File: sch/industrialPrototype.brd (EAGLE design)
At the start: 160 x 100 mm, 13 parts, among them IC1 LD1117V33C, U1 PIC16F1825-I/SL

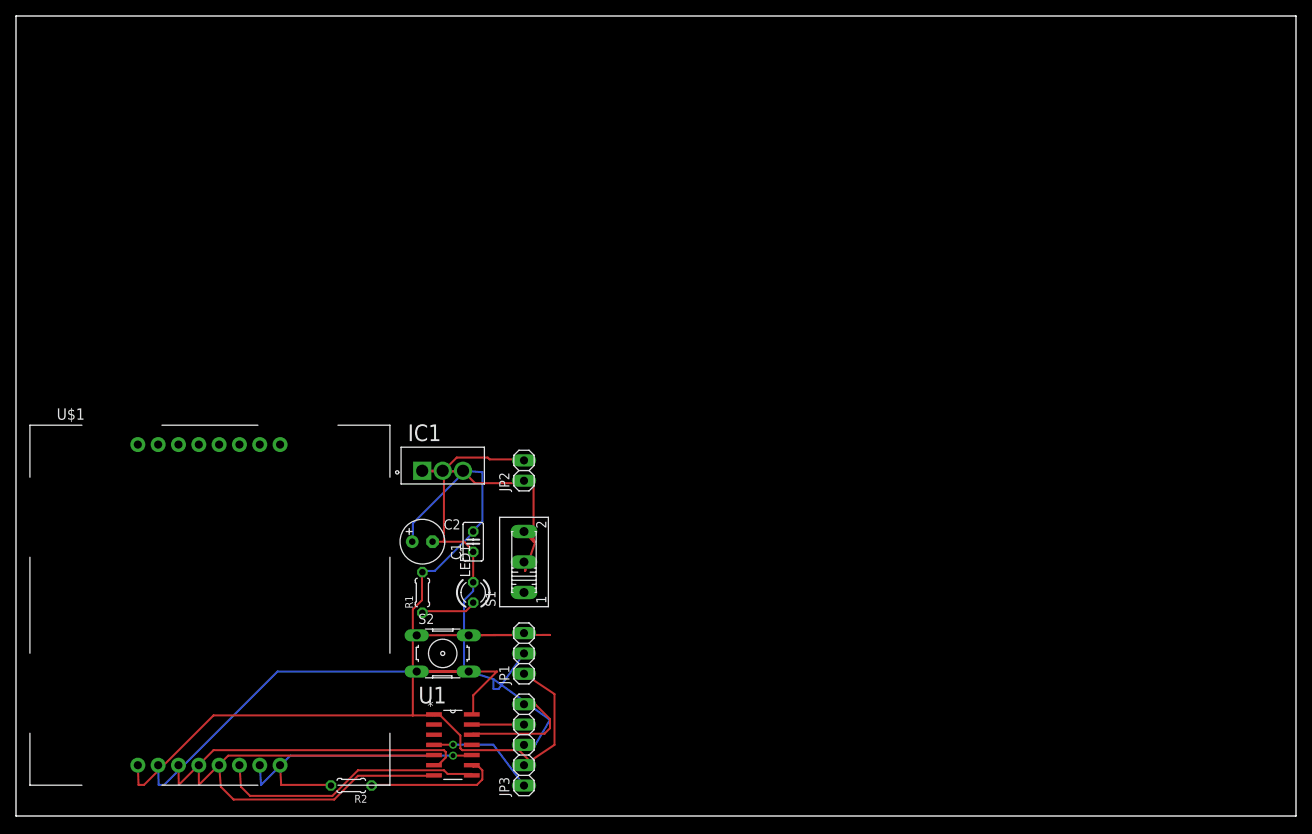
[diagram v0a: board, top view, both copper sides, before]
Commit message: Final Version of the Schematic and Board
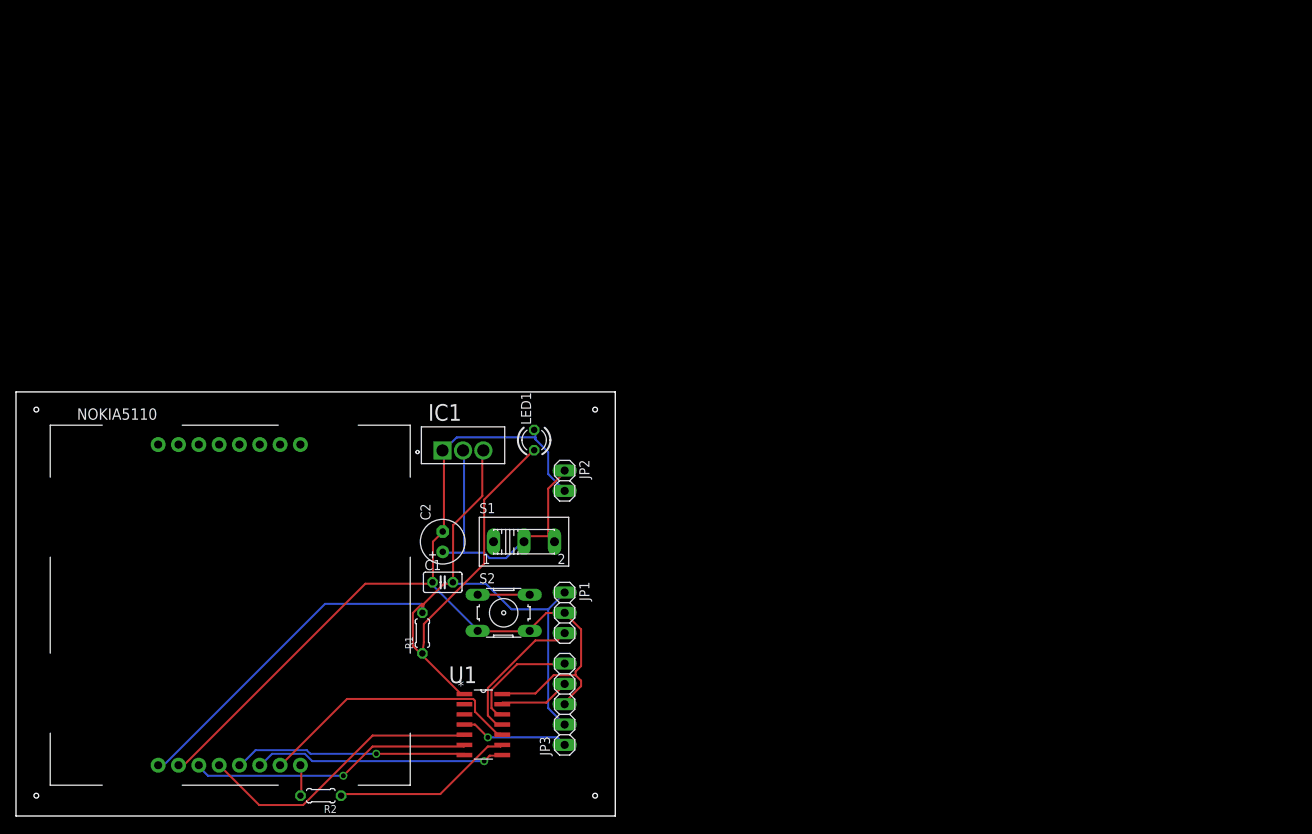
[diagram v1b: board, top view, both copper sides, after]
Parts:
- removed U$1: NOKIA5110, CustomLib:NOKIA5110
- added NOKIA5110: NOKIA5110, CustomLib:NOKIA5110
- moved LED1 20.5 mm to (64.8, 47.0)
- moved S2 9.16 mm to (61.0, 25.4)
- moved JP3 7.18 mm to (68.6, 14.0)
- moved JP1 7.18 mm to (68.6, 25.4), turned to 270 degrees
- moved C1 6.35 mm to (53.3, 29.2), turned to 0 degrees
- moved JP2 5.24 mm to (68.6, 41.9), turned to 270 degrees
- moved R1 5.08 mm to (50.8, 22.9)
- moved U1 4.58 mm to (58.4, 11.4)
- moved R2 4.02 mm to (38.1, 2.54)
- moved IC1 3.59 mm to (58.4, 47.0)
- moved C2 2.54 mm to (53.3, 34.3), turned to 90 degrees
- moved S1 2.54 mm to (63.5, 34.3), turned to 0 degrees
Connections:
- net !RST!: now also NOKIA5110.B4; no longer U$1.B4
- net !SCE!: now also NOKIA5110.B3; no longer U$1.B3
- net 3V3: now also NOKIA5110.B1; no longer U$1.B1
- net D/C: now also NOKIA5110.B5; no longer U$1.B5
- net DN(MOSI): now also NOKIA5110.B6; no longer U$1.B6
- net GND: now also NOKIA5110.B2; no longer U$1.B2
- net LED: now also NOKIA5110.B8; no longer U$1.B8
- net SCLK: now also NOKIA5110.B7; no longer U$1.B7
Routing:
- net N$1: track 6.97 -> 31.2 mm
- net !MCLK!: track 26.8 -> 6.50 mm
- net GND: track 142.4 -> 124.2 mm
- net 1WIRE_DS18B20: track 0.00 -> 18.1 mm
- net VBAT: track 44.6 -> 38.6 mm
- net N$3: track 16.9 -> 22.8 mm
- net LED: track 8.73 -> 3.87 mm
- net !SCE!: track 40.3 -> 35.5 mm, vias 0 -> 1
- net SCLK: track 30.4 -> 33.8 mm, vias 1 -> 0
- net !RST!: track 33.4 -> 36.4 mm
- net ICSPDAT: track 6.53 -> 8.97 mm
- net DN(MOSI): track 33.7 -> 31.6 mm, vias 0 -> 1
- net D/C: track 31.2 -> 29.2 mm, vias 0 -> 1
- net 3V3: track 113.0 -> 113.8 mm
- net ICSPCLK: track 15.3 -> 14.5 mm
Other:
- board size 160 x 100 mm -> 74.9 x 53 mm
